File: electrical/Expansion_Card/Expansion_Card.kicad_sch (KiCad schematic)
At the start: 39 parts, among them J1 Micro_SD_Card_Det2, J2 SD_Card_Receptacle, P1 USB_C_Plug_USB2.0, U1 AP2112K-3.3, U2 USB2660I-JZX-03, X1 24MHz ASCO

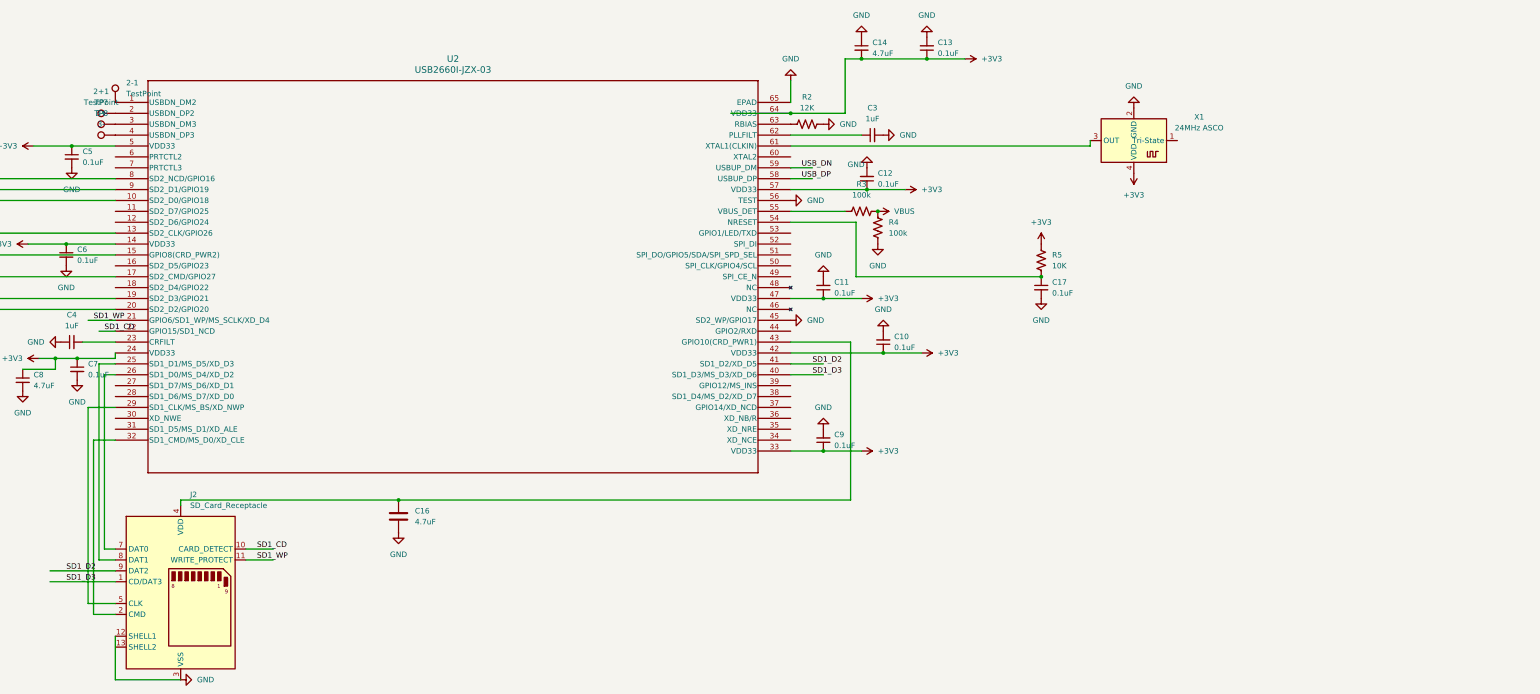
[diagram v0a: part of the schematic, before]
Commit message: I have regrets
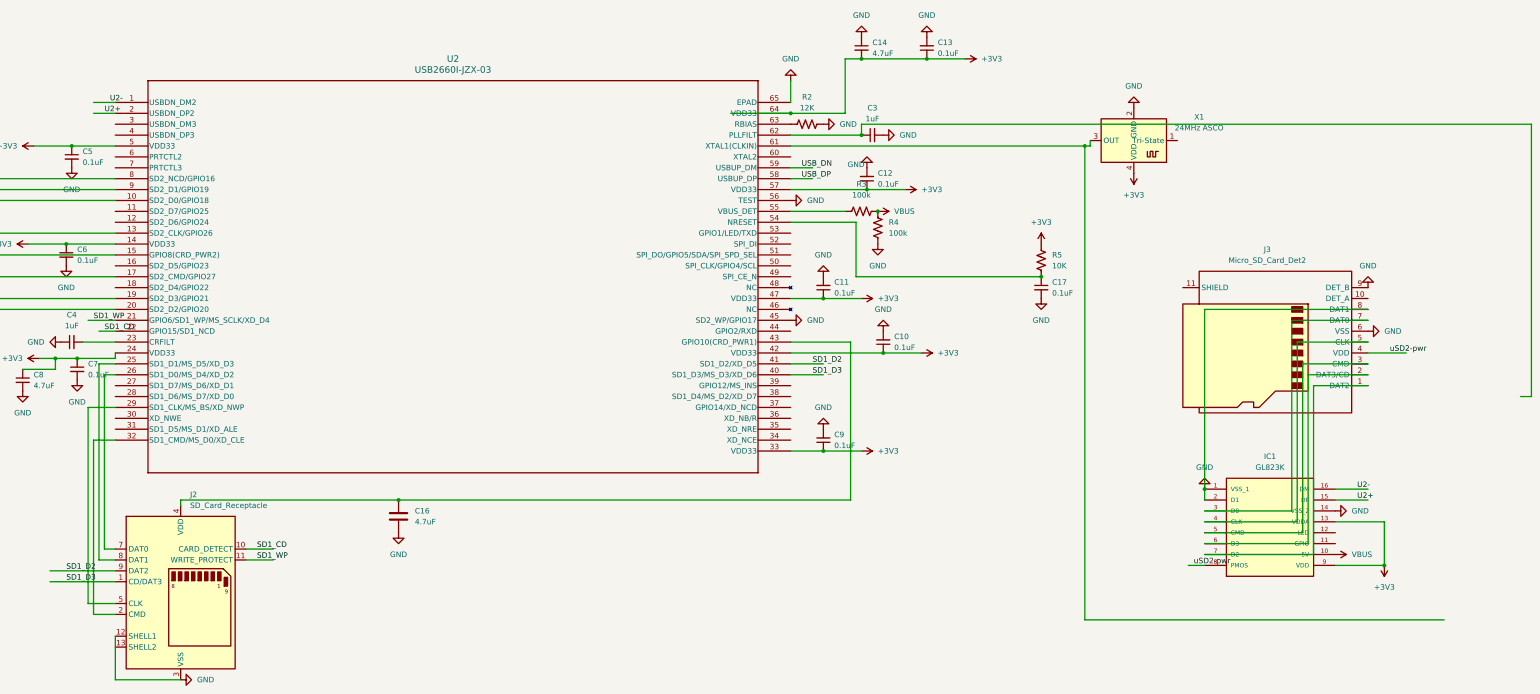
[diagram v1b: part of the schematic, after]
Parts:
- removed 2+1, 2-1: TestPoint, TestPoint:TestPoint_Pad_2.0x2.0mm, symbol Connector:TestPoint
- removed TP7: 3+, TestPoint:TestPoint_Pad_2.0x2.0mm, symbol Connector:TestPoint
- removed TP8: 3-, TestPoint:TestPoint_Pad_2.0x2.0mm, symbol Connector:TestPoint
- added IC1: GL823K, Expansion_Card:SOP64P600X175-16N, symbol GL823K:GL823K
- added J3: Micro_SD_Card_Det2, Connector_Card:microSD_HC_Molex_104031-0811, symbol Connector:Micro_SD_Card_Det2
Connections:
- net +3V3: now also IC1.13 (VDDA), IC1.9 (VDD)
- net GND: now also IC1.1 (VSS_1), IC1.14 (VSS_2), IC1.2 (D1), J3.6 (VSS), J3.8 (DAT1), J3.9 (DET_B)
- net VBUS: now also IC1.10 (5V)
- net U2+: now reaches U2.2 (USBDN_DP2)
- net U2+: now also IC1.15 (DP)
- net U2-: now reaches U2.1 (USBDN_DM2)
- net U2-: now also IC1.16 (DM)
- new net: IC1.3 (D0), J3.7 (DAT0)
- new net: IC1.4 (CLK), J3.5 (CLK)
- new net: IC1.5 (CMD), J3.3 (CMD)
- new net: IC1.6 (D3), J3.2 (DAT3/CD)
- new net: IC1.7 (D2), J3.1 (DAT2)
- new net uSD2-pwr: IC1.8 (PMOS), J3.4 (VDD)
